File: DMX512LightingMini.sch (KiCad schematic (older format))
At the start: 1 part

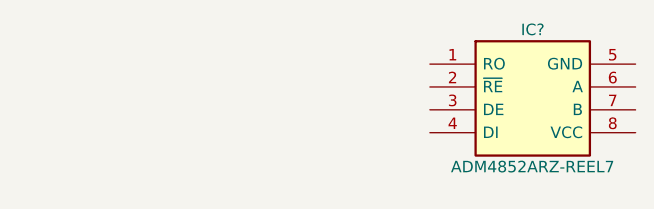
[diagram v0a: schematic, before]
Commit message: * 部品配置開始
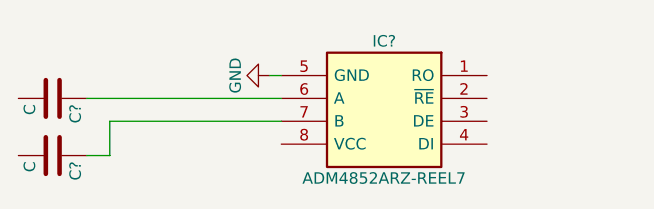
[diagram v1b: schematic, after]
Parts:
- added C? (x2): C, symbol C
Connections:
- net GND: now reaches IC?.5 (GND)
- net at IC?.6 (A): now also C?.1
- net at IC?.7 (B): now also C?.1
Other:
- moved on the sheet: IC?
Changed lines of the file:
@@
 LIBS:valves
 LIBS:SamacSys_Parts
+LIBS:DMX512LightingMini-cache
 EELAYER 25 0
 EELAYER END
@@
 L ADM4852ARZ-REEL7 IC?
 U 1 1 599C318A
-P 5150 3900
-F 0 "IC?" H 5600 4050 50  0000 C CNN
-F 1 "ADM4852ARZ-REEL7" H 5600 3450 50  0000 C CNN
-F 2 "SOIC127P600X175-8N" H 5600 3350 50  0001 C CNN
-F 3 "" H 5600 3250 50  0001 C CNN
-F 4 "Transceivers" H 5600 3150 50  0001 C CNN "Description"
-F 5 "RS" H 5600 3050 50  0001 C CNN "Supplier_Name"
-F 6 "" H 5600 2950 50  0001 C CNN "RS Part Number"
-F 7 "Analog Devices" H 5600 2850 50  0001 C CNN "Manufacturer_Name"
-F 8 "ADM4852ARZ-REEL7" H 5600 2750 50  0001 C CNN "Manufacturer_Part_Number"
-F 9 "" H 5600 2650 50  0001 C CNN "Allied_Number"
-F 10 "" H 5600 2550 50  0001 C CNN "Other Part Number"
-F 11 "" H 5900 2450 50  0001 C CNN "Height"
-	1    5150 3900
-	1    0    0    -1
+P 5400 3950
+F 0 "IC?" H 5850 4100 50  0000 C CNN
+F 1 "ADM4852ARZ-REEL7" H 5850 3500 50  0000 C CNN
+F 2 "SOIC127P600X175-8N" H 5850 3400 50  0001 C CNN
+F 3 "" H 5850 3300 50  0001 C CNN
+F 4 "Transceivers" H 5850 3200 50  0001 C CNN "Description"
+F 5 "RS" H 5850 3100 50  0001 C CNN "Supplier_Name"
+F 6 "Analog Devices" H 5850 2900 50  0001 C CNN "Manufacturer_Name"
+F 7 "ADM4852ARZ-REEL7" H 5850 2800 50  0001 C CNN "Manufacturer_Part_Number"
+	1    5400 3950
+	-1   0    0    -1
 $EndComp
+$Comp
+L C C?
+U 1 1 599C34D2
+P 3500 4050
+F 0 "C?" H 3525 4150 50  0000 L CNN
+F 1 "C" H 3525 3950 50  0000 L CNN
+F 2 "" H 3538 3900 50  0001 C CNN
+F 3 "" H 3500 4050 50  0001 C CNN
+	1    3500 4050
+	0    1    1    0
+$EndComp
+$Comp
+L C C?
+U 1 1 599C360D
+P 3500 4300
+F 0 "C?" H 3525 4400 50  0000 L CNN
+F 1 "C" H 3525 4200 50  0000 L CNN
+F 2 "" H 3538 4150 50  0001 C CNN
+F 3 "" H 3500 4300 50  0001 C CNN
+	1    3500 4300
+	0    1    1    0
+$EndComp
+$Comp
+L GND #PWR?
+U 1 1 599C37CE
+P 4450 3950
+F 0 "#PWR?" H 4450 3700 50  0001 C CNN
+F 1 "GND" H 4450 3800 50  0000 C CNN
+F 2 "" H 4450 3950 50  0001 C CNN
+F 3 "" H 4450 3950 50  0001 C CNN
+	1    4450 3950
+	0    1    1    0
+$EndComp
+Wire Wire Line
+	4450 3950 4500 3950
+Wire Wire Line
+	4500 4050 3650 4050
+Wire Wire Line
+	3650 4300 3750 4300
+Wire Wire Line
+	3750 4300 3750 4150
+Wire Wire Line
+	3750 4150 4500 4150
 $EndSCHEMATC
